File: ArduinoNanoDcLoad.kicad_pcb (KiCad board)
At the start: 2 copper layers, 200 x 100 mm, 49 parts, among them CON1 BARREL_JACK, P1 DCLOAD+, P2 DCLOAD-, P3 CONN_01X15, P4 CONN_01X15, Q1 IRFP250N, U1 LMC6484, U2 LM7812, U3 LM317T

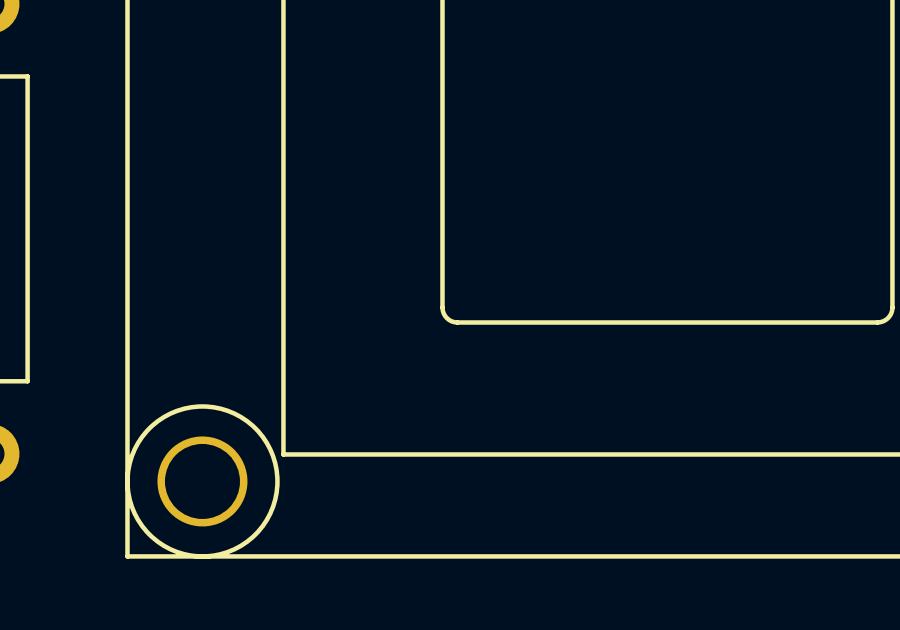
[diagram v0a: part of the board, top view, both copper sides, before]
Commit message: update
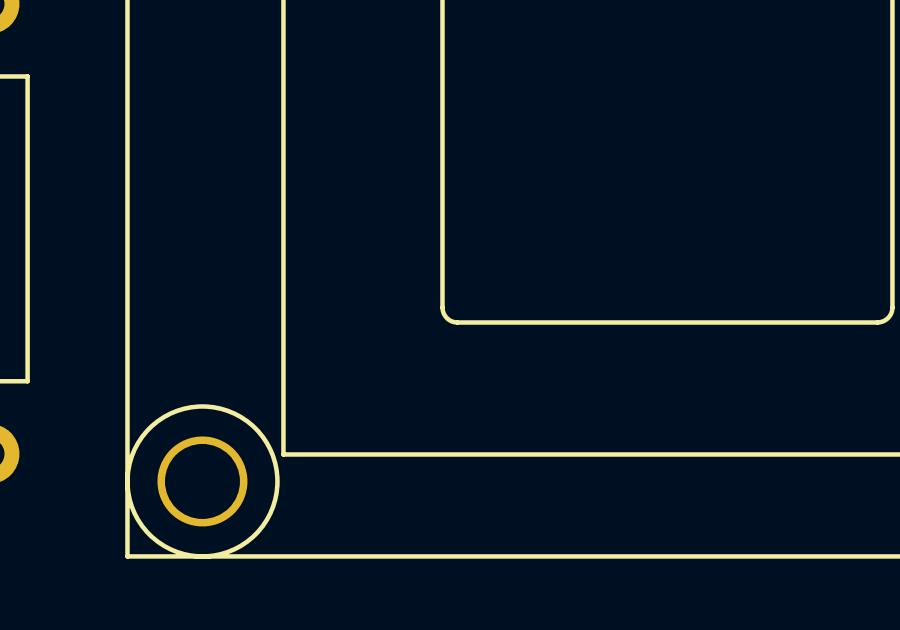
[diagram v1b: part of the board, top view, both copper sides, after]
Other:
- net class Default removed
- net class HeavyLoadNet removed
